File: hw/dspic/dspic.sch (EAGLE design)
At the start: 20 parts, among them Q1 8MH

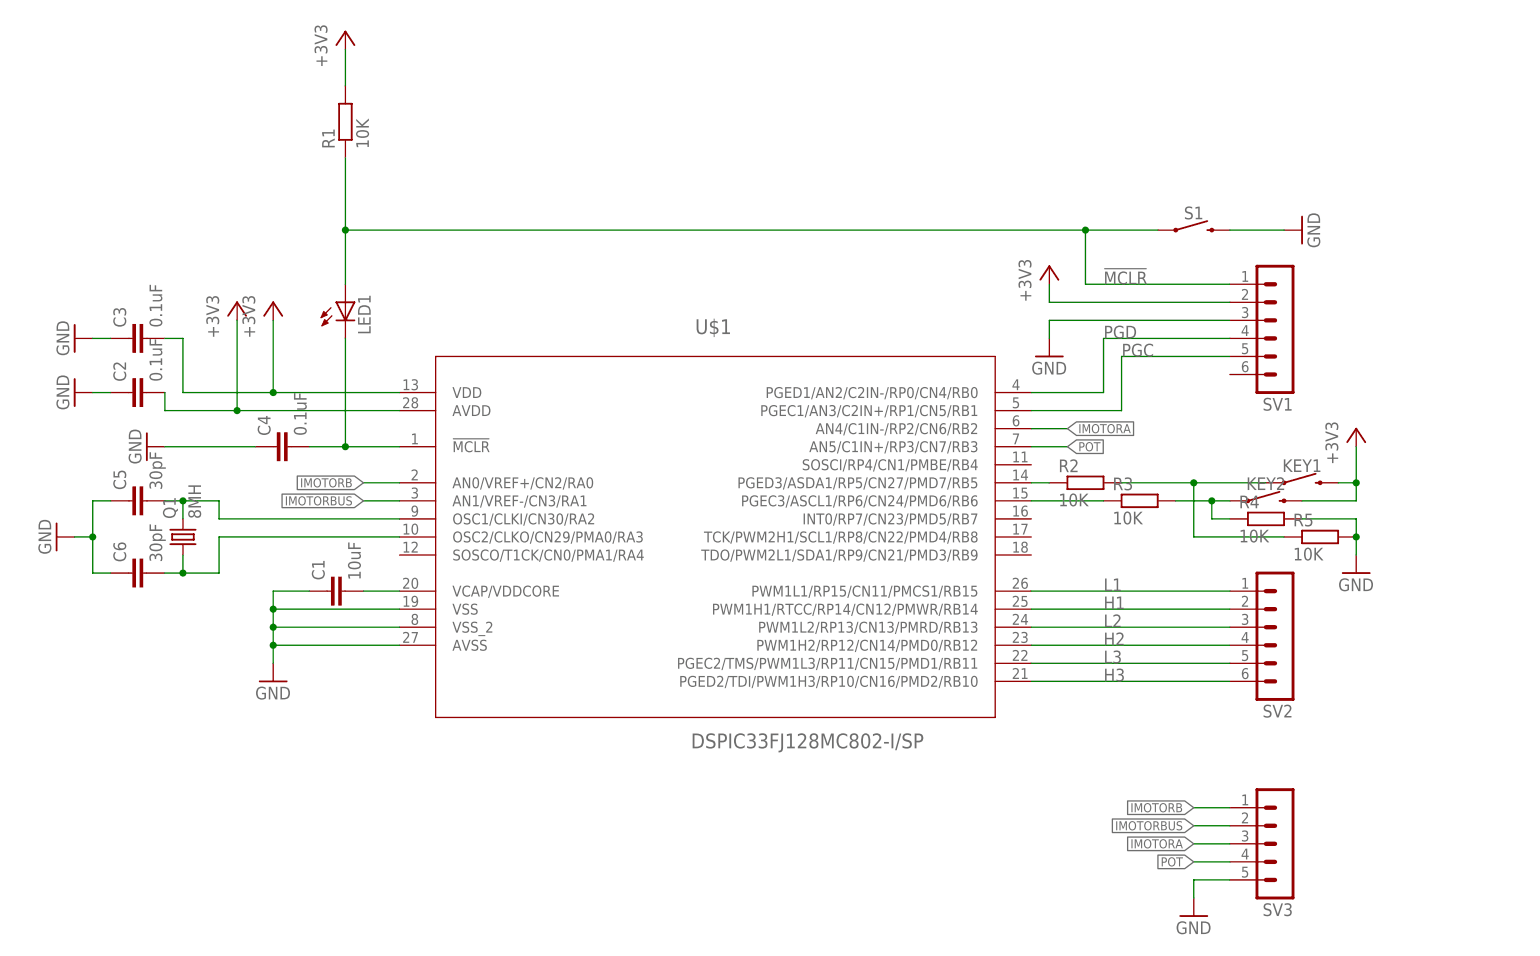
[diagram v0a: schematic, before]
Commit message: dspic brd
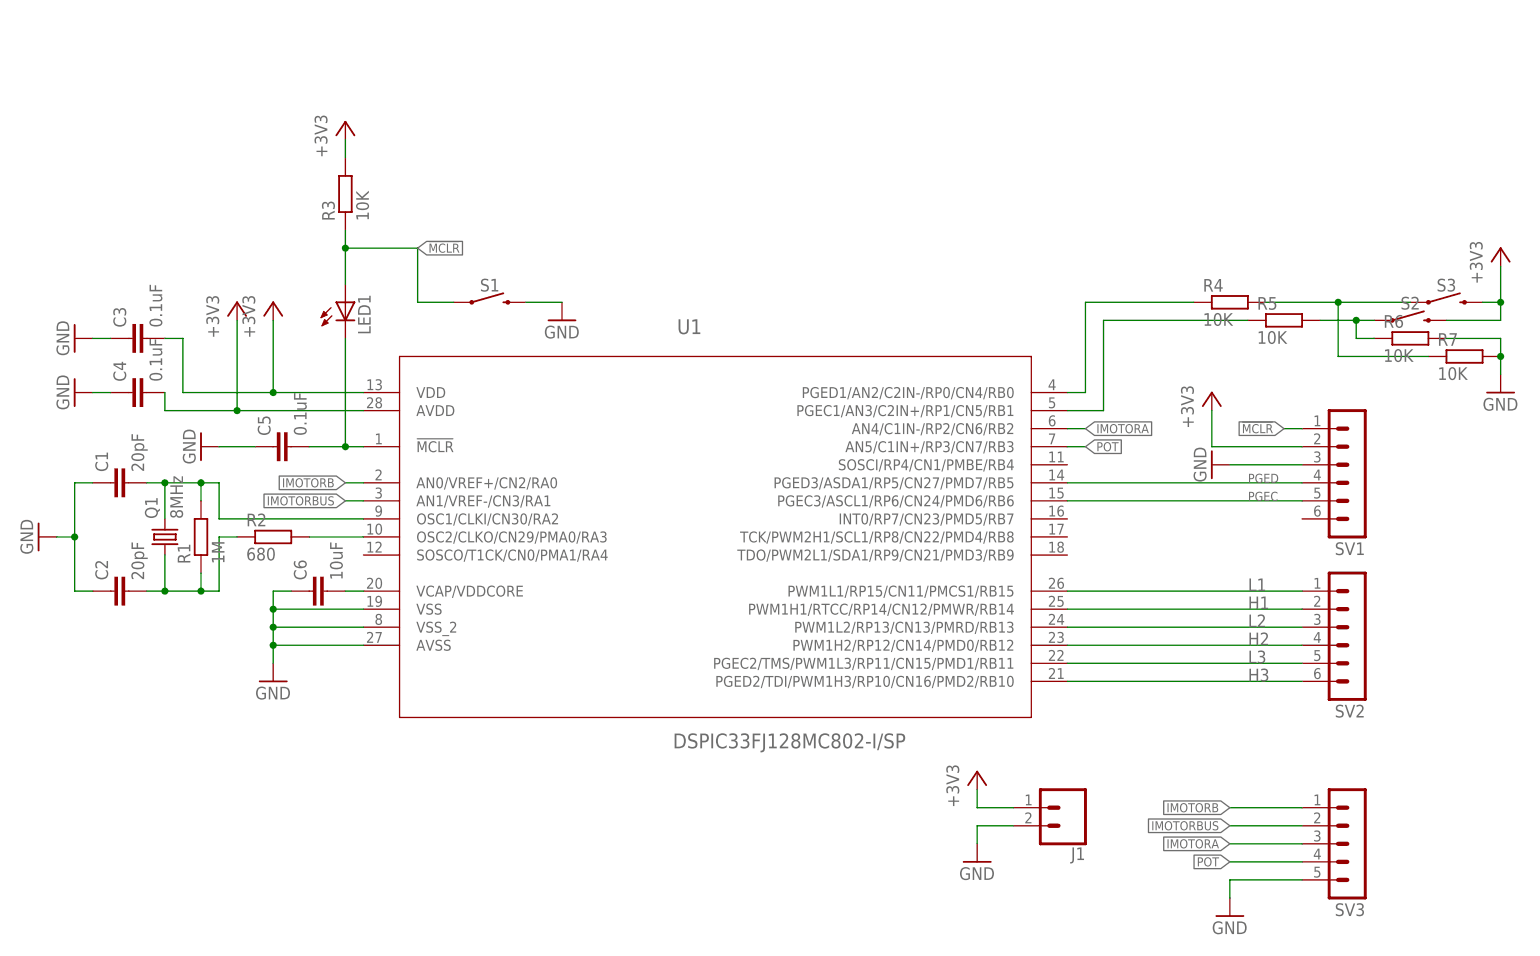
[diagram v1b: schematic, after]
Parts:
- removed KEY1, KEY2: MOMENTARY-SWITCH-SPST-PTH-6.0MM, SparkFun-Switches:MOMENTARY-SWITCH-SPST-PTH-6.0MM
- removed U$1: DSPIC33FJ128MC802-I/SP, Microchip-DSPIC33FJ128MC802-I_SP:DSPIC33FJ128MC802-I/SP
- added J1: (no value), SparkFun-Connectors:CONN_02
- added R6, R7: 10K, resistor:R-EU_0207/10
- added S2, S3: MOMENTARY-SWITCH-SPST-PTH-6.0MM, SparkFun-Switches:MOMENTARY-SWITCH-SPST-PTH-6.0MM
- added U1: DSPIC33FJ128MC802-I/SP, Microchip-DSPIC33FJ128MC802-I_SP:DSPIC33FJ128MC802-I/SP
- C1: value 10uF -> 20pF
- C2: value 0.1uF -> 20pF
- C5: value 30pF -> 0.1uF
- C6: value 30pF -> 10uF
- Q1: value 8MH -> 8MHz; device crystal:CRYSTALHC49U70 -> crystal:CRYSTALHC49S
- R1: value 10K -> 1M
- R2: value 10K -> 680
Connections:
- removed net N$5: R2.1, U$1.PGED3/ASDA1/RP5/CN27/PMD7/RB5
- removed net N$6: R3.1, U$1.PGEC3/ASCL1/RP6/CN24/PMD6/RB6
- removed net PGC: SV1.5, U$1.PGEC1/AN3/C2IN+/RP1/CN5/RB1
- removed net PGD: SV1.4, U$1.PGED1/AN2/C2IN-/RP0/CN4/RB0
- new net N$10: R5.1, U1.PGEC1/AN3/C2IN+/RP1/CN5/RB1
- new net N$11: R4.1, U1.PGED1/AN2/C2IN-/RP0/CN4/RB0
- new net N$9: R2.2, U1.OSC2/CLKO/CN29/PMA0/RA3
- new net PGEC: SV1.5, U1.PGEC3/ASCL1/RP6/CN24/PMD6/RB6
- new net PGED: SV1.4, U1.PGED3/ASDA1/RP5/CN27/PMD7/RB5
- net !MCLR!: now also R3.1; no longer R1.1
- net +3V3: now also C4.2, J1.1, R3.2, S2.2, S3.2, U1.AVDD, U1.VDD; no longer C2.2, KEY1.2, KEY2.2, R1.2, U$1.AVDD, U$1.VDD
- net GND: now also J1.2, R6.2, R7.2, U1.AVSS, U1.VSS, U1.VSS_2; no longer R4.2, R5.2, U$1.AVSS, U$1.VSS, U$1.VSS_2
- net H1: now also U1.PWM1H1/RTCC/RP14/CN12/PMWR/RB14; no longer U$1.PWM1H1/RTCC/RP14/CN12/PMWR/RB14
- net H2: now also U1.PWM1H2/RP12/CN14/PMD0/RB12; no longer U$1.PWM1H2/RP12/CN14/PMD0/RB12
- net H3: now also U1.PGED2/TDI/PWM1H3/RP10/CN16/PMD2/RB10; no longer U$1.PGED2/TDI/PWM1H3/RP10/CN16/PMD2/RB10
- net IMOTORA: now also U1.AN4/C1IN-/RP2/CN6/RB2; no longer U$1.AN4/C1IN-/RP2/CN6/RB2
- net IMOTORB: now also U1.AN0/VREF+/CN2/RA0; no longer U$1.AN0/VREF+/CN2/RA0
- net IMOTORBUS: now also U1.AN1/VREF-/CN3/RA1; no longer U$1.AN1/VREF-/CN3/RA1
- net L1: now also U1.PWM1L1/RP15/CN11/PMCS1/RB15; no longer U$1.PWM1L1/RP15/CN11/PMCS1/RB15
- net L2: now also U1.PWM1L2/RP13/CN13/PMRD/RB13; no longer U$1.PWM1L2/RP13/CN13/PMRD/RB13
- net L3: now also U1.PGEC2/TMS/PWM1L3/RP11/CN15/PMD1/RB11; no longer U$1.PGEC2/TMS/PWM1L3/RP11/CN15/PMD1/RB11
- net N$1: now also C6.2, U1.VCAP/VDDCORE; no longer C1.2, U$1.VCAP/VDDCORE
- net N$2: now also C5.2, U1.!MCLR!; no longer C4.2, U$1.!MCLR!
- net N$3: now also R4.2, R7.1, S3.1; no longer KEY1.1, R2.2, R5.1
- net N$4: now also R5.2, R6.1, S2.1; no longer KEY2.1, R3.2, R4.1
- net N$7: now also C1.2, R1.2, U1.OSC1/CLKI/CN30/RA2; no longer C5.2, U$1.OSC1/CLKI/CN30/RA2
- net N$8: now also C2.2, R1.1, R2.1; no longer C6.2, U$1.OSC2/CLKO/CN29/PMA0/RA3
- net POT: now also U1.AN5/C1IN+/RP3/CN7/RB3; no longer U$1.AN5/C1IN+/RP3/CN7/RB3
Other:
- moved on the sheet: C1, C2, C4, C5, C6, Q1, R1, R2, R3, R4, R5, S1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
